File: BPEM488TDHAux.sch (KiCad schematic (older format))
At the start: 100 parts, among them J1 Conn_01x02, J2 Conn_02x18_Odd_Even, J3 DB15_Female, J4 DB15_Female, Q1 ZTX450, Q10 ZTX450, Q11 ZTX450, Q12 ZTX450, Q13 ZTX450, Q14 ZTX450, Q15 ZTX450, Q16 ZTX450, Q17 ZTX450, Q18 ZTX450, Q19 ZTX450, Q2 ZTX450, Q20 ZTX450, Q21 ZTX450, Q22 ZTX450, Q23 ZTX450, Q24 ZTX450, Q25 ZTX450, Q3 ZTX450, Q4 ZTX450, Q5 ZTX450, Q6 ZTX450, Q7 ZTX450, Q8 ZTX450, Q9 ZTX450, U1 LD1085V50, U2 L7808ABV

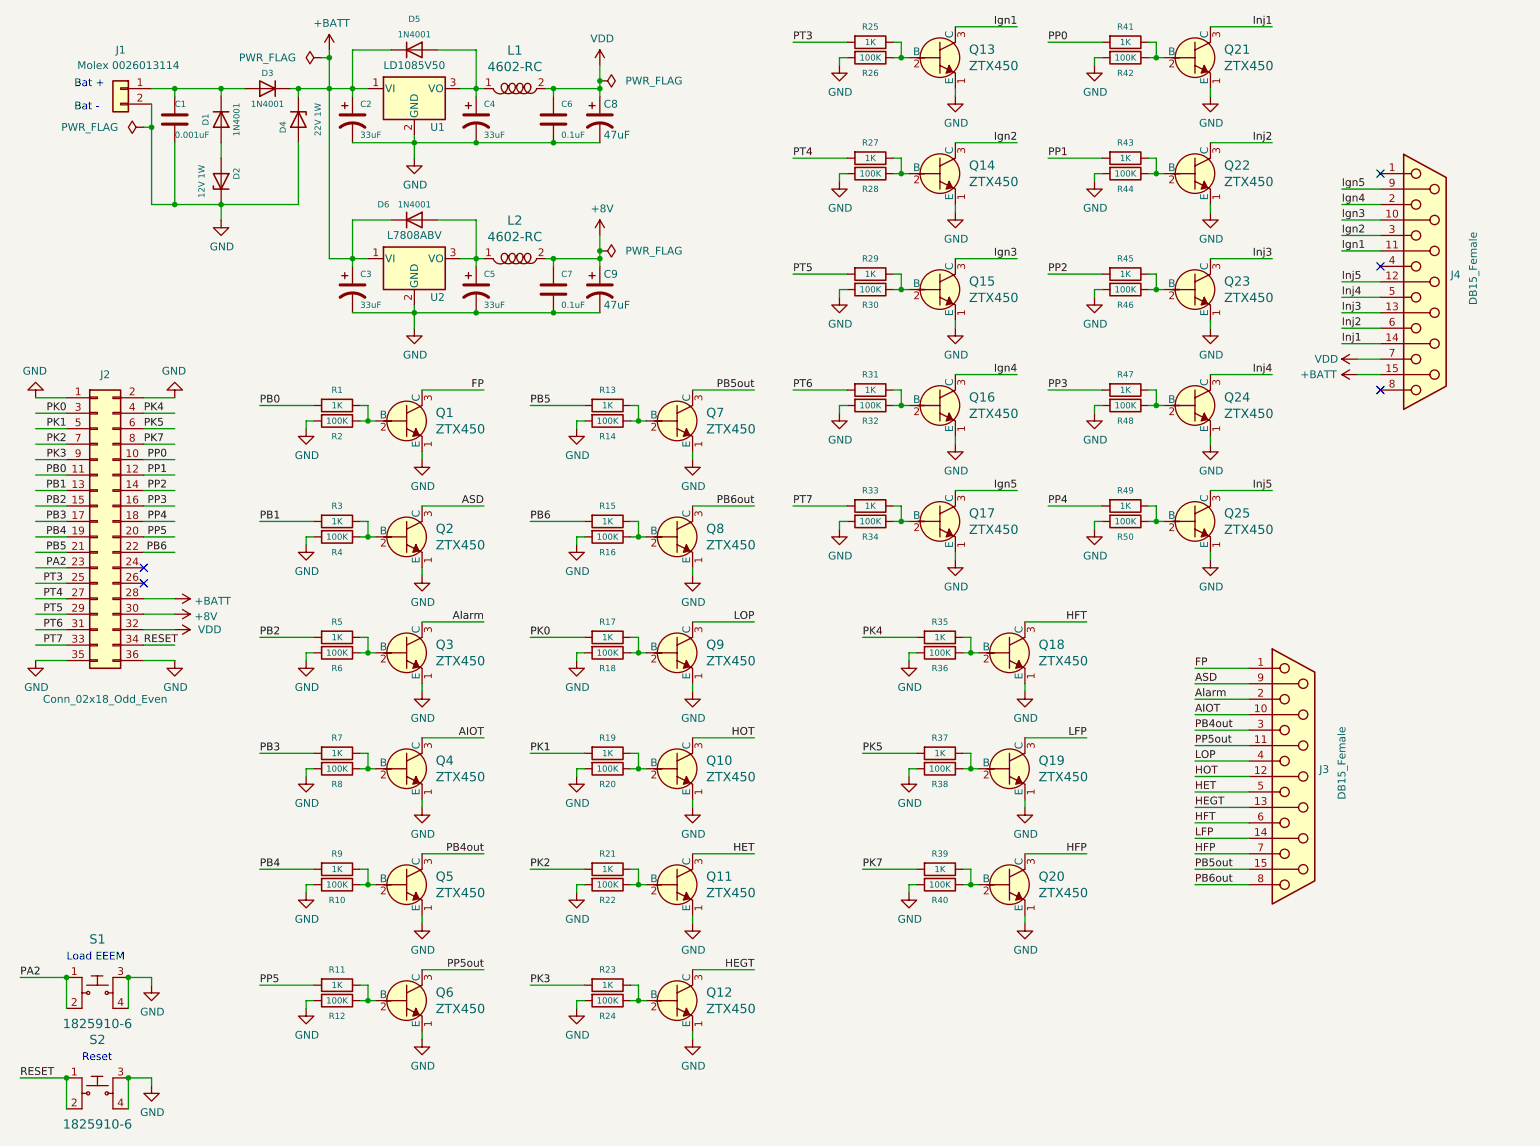
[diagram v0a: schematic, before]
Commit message: Add files via upload
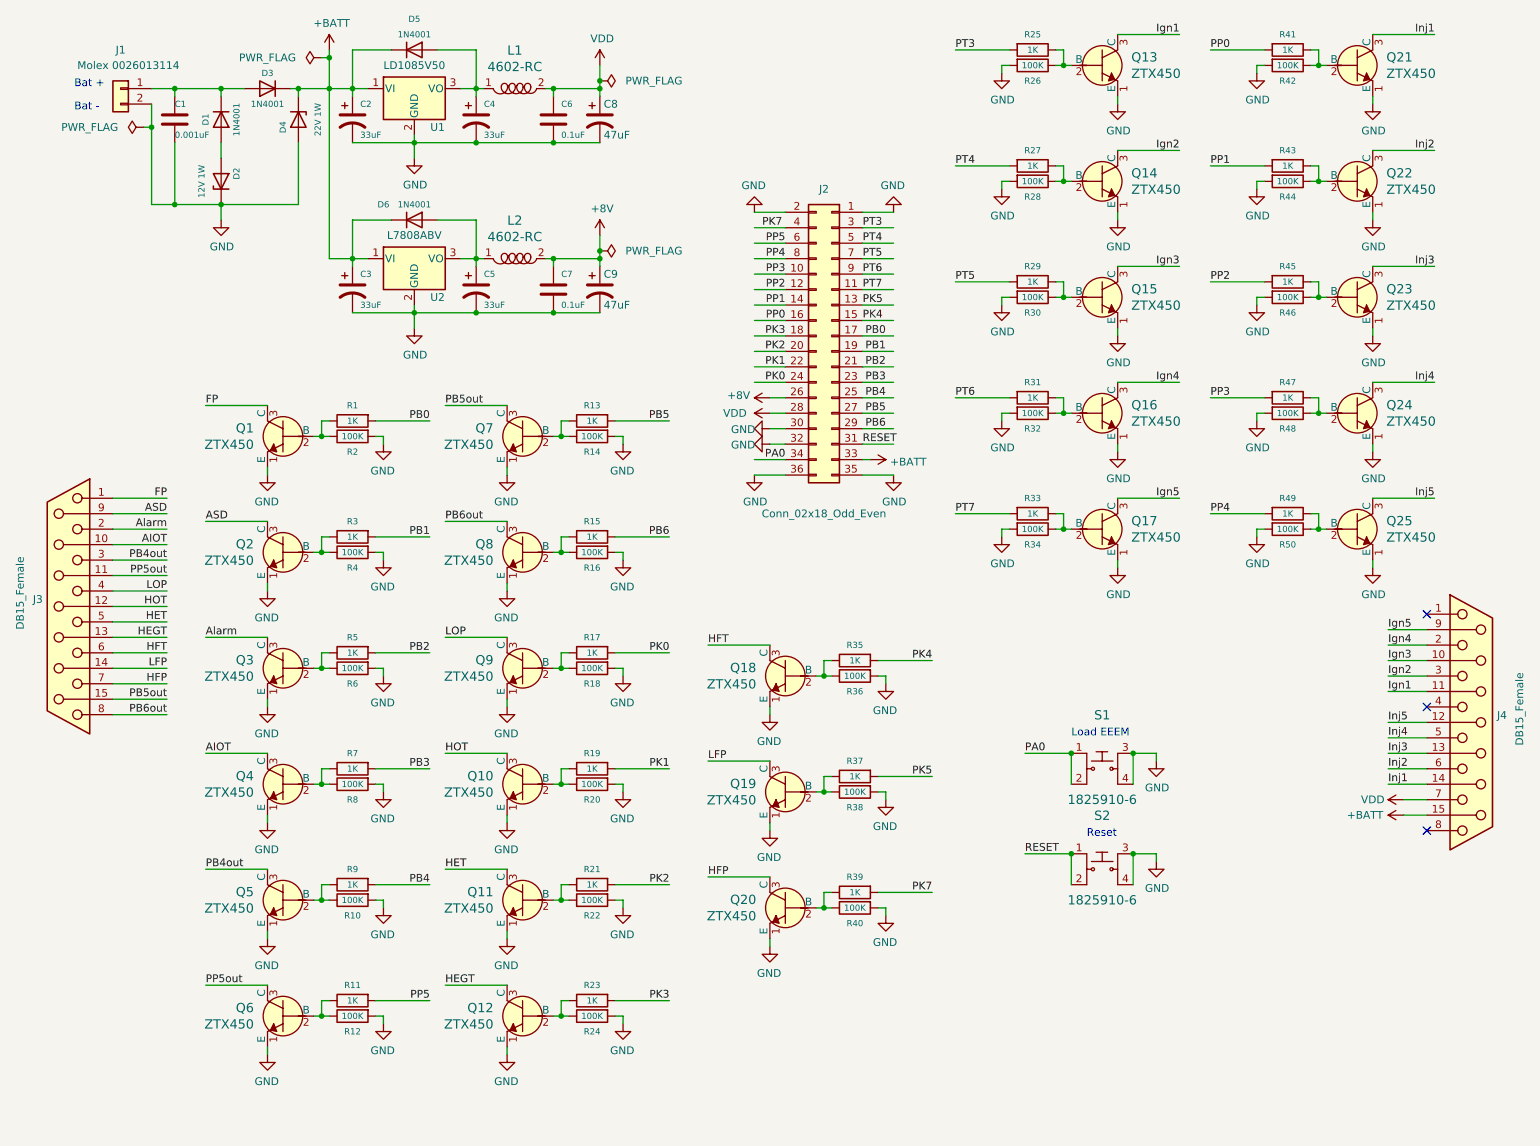
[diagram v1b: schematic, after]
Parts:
- J2: footprint Connector_PinHeader_2.54mm:PinHeader_2x18_P2.54mm_Vertical -> Connector_PinSocket_2.54mm:PinSocket_2x18_P2.54mm_Vertical
- J3, J4: Digikey 609-1499-ND -> A32123-ND; Mfg D15S33E4GX00LF -> 5747845-6
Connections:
- net labels added: PA0
- net labels removed: PA2
- wire segments 362 -> 364
- no-connect marks 5 -> 3
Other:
- moved on the sheet: J2, J3, J4, Q1, Q10, Q11, Q12, Q13, Q14, Q15, Q16, Q17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
